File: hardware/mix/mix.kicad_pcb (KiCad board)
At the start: 2 copper layers, 54.6 x 30.5 mm, 6 parts, among them T1 ETC4-1-2TR, T2 ETC4-1-2TR

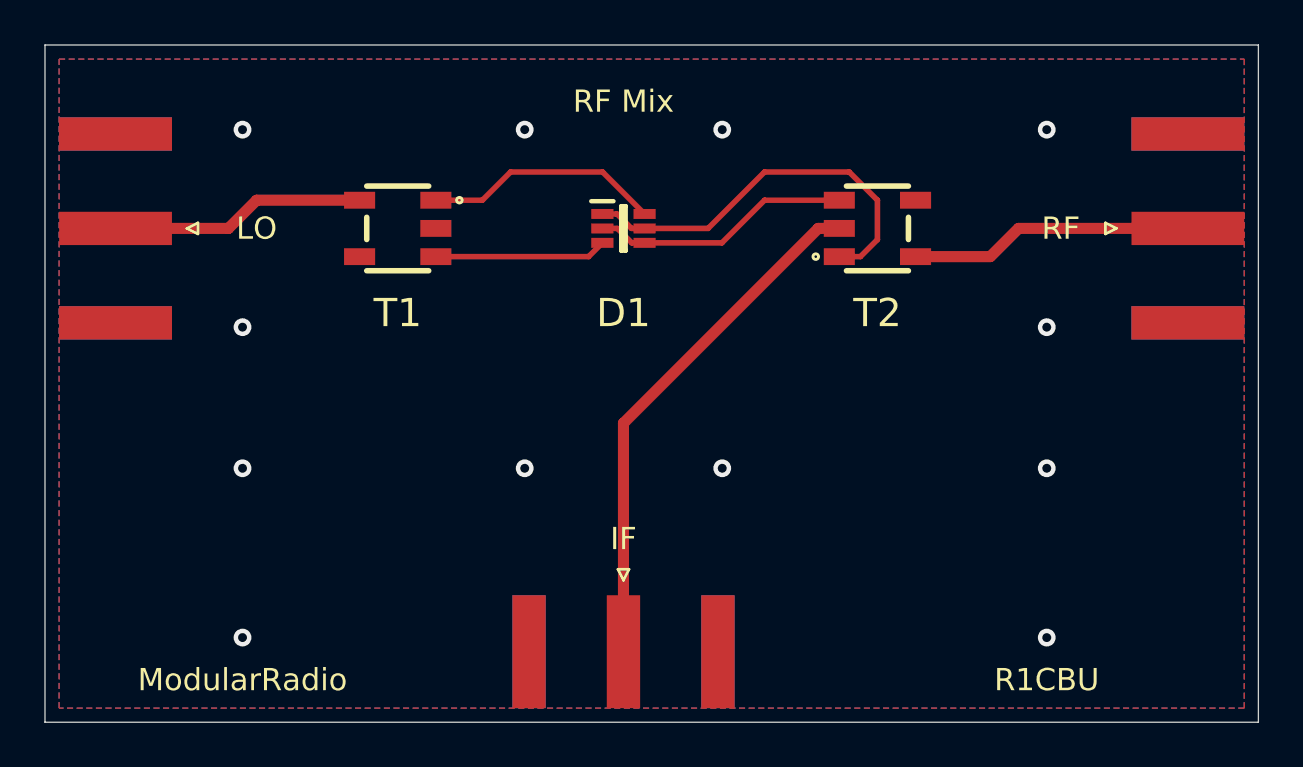
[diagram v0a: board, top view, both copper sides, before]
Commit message: Optimize Quad DDC, Gerber files
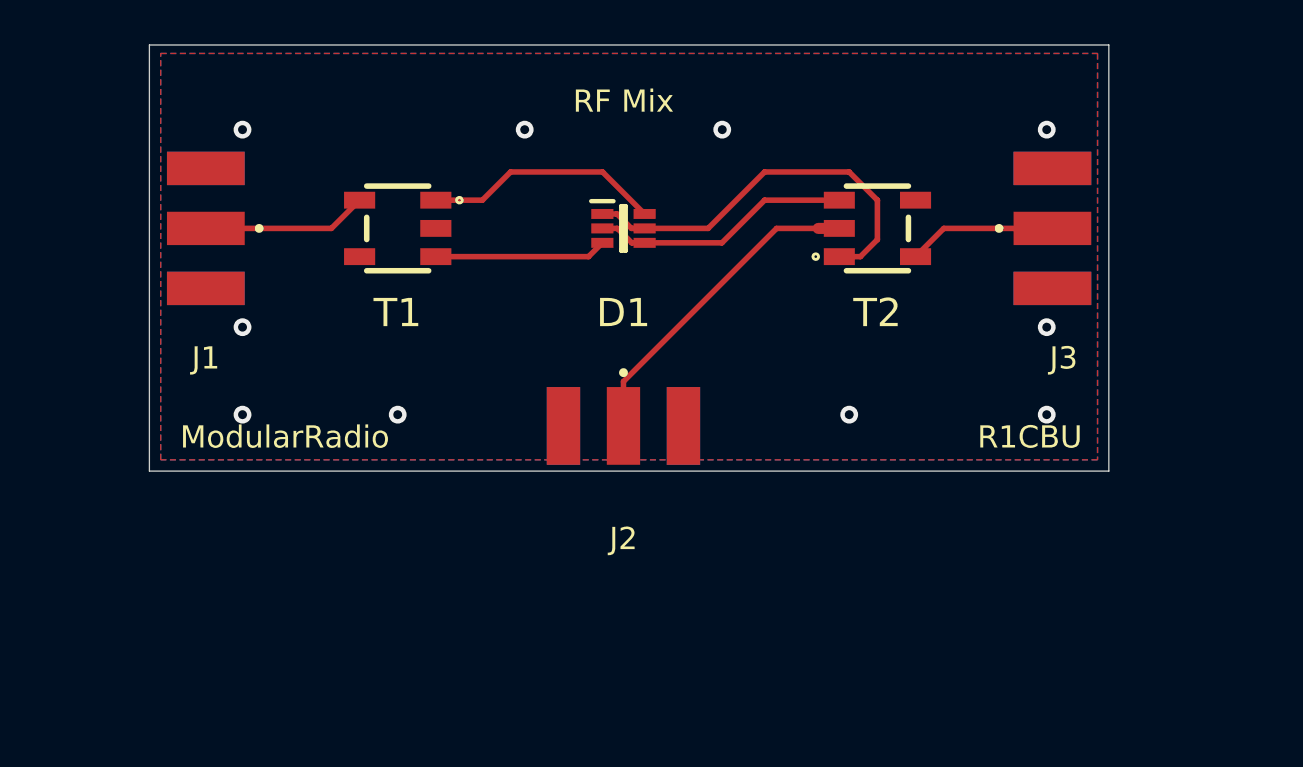
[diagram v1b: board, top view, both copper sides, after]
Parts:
- J1: renamed from LO; footprint Connector_Coaxial:SMA_Amphenol_132289_EdgeMount -> kicad:RFSOLUTIONS_CON-SMA-EDGE-S
- J2: renamed from IF; footprint Connector_Coaxial:SMA_Amphenol_132289_EdgeMount -> kicad:RFSOLUTIONS_CON-SMA-EDGE-S
- J3: renamed from RF; footprint Connector_Coaxial:SMA_Amphenol_132289_EdgeMount -> kicad:RFSOLUTIONS_CON-SMA-EDGE-S
- moved J2 10.2 mm to (147.3, 101.6), turned to 90 degrees
- moved J3 6.10 mm to (166.6, 92.7), turned to 180 degrees
- moved J1 4.06 mm to (128.5, 92.7), turned to 0 degrees
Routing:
- net Net-(J2-Pad1): track 23.6 -> 15.5 mm
- net Net-(J3-Pad1): track 12.8 -> 6.69 mm
- net Net-(J1-Pad1): track 11.5 -> 7.45 mm
- net GND: vias 12 -> 10
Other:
- board size 54.6 x 30.5 mm -> 43.2 x 19.2 mm
